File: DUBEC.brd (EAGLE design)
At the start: 40 x 21.4 mm, 72 parts

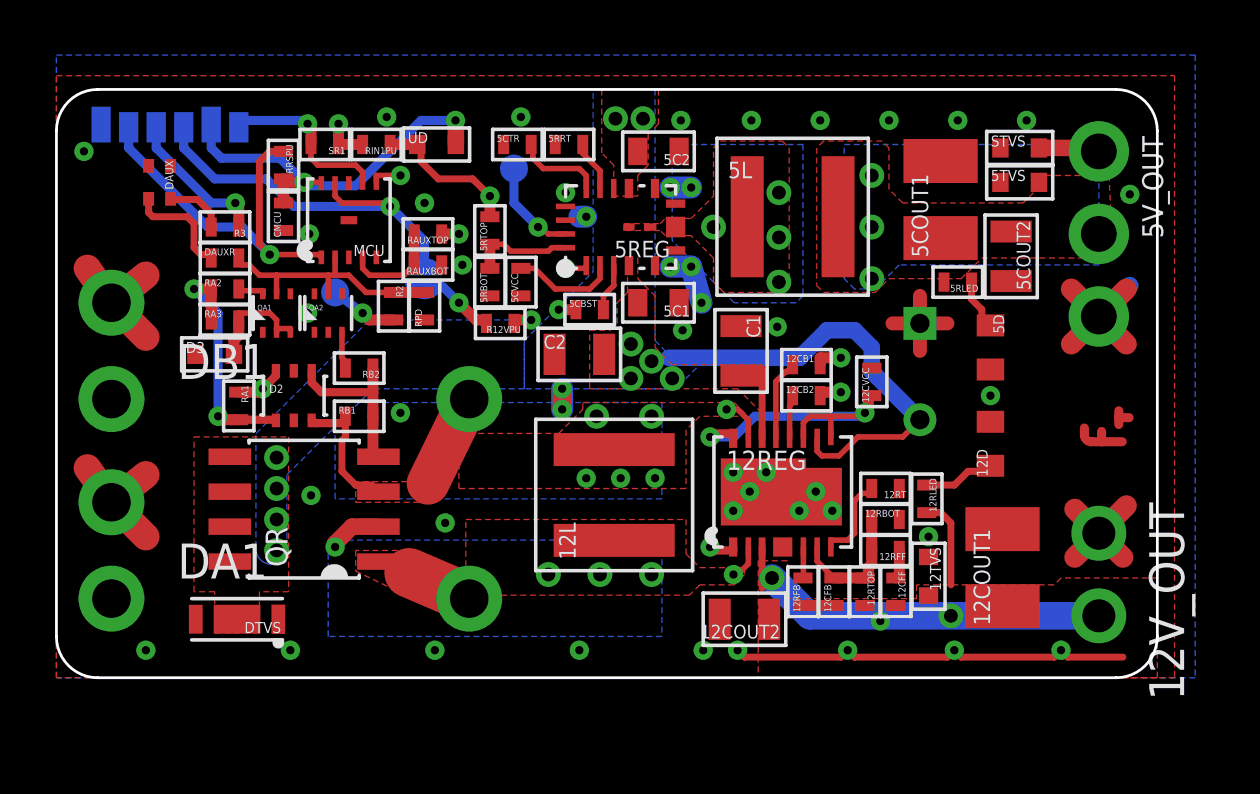
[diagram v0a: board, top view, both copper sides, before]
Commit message: Bored wanking
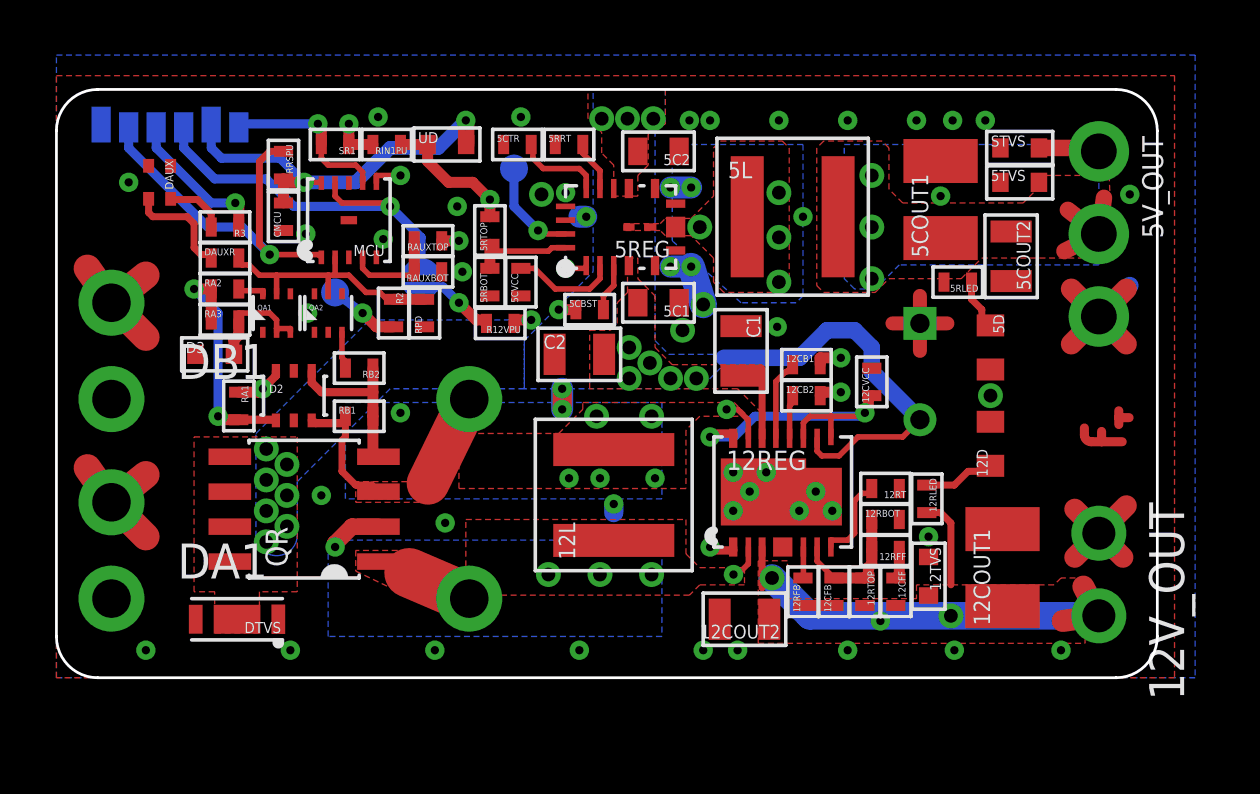
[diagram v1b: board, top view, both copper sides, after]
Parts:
- C1, C2: value 22uF -> (none)
- moved RIN1PU 0.38 mm to (12.0, 19.4)
- moved SR1 0.38 mm to (10.1, 19.4)
- moved UD 0.38 mm to (14.2, 19.4)
- moved R2 0.25 mm to (12.2, 13.2)
- moved RAUXBOT 0.25 mm to (13.5, 14.8)
- moved RAUXTOP 0.25 mm to (13.5, 15.9)
- moved RPD 0.25 mm to (13.4, 13.2)
- moved SJ1 0.12 mm to (13.2, 14.5)
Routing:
- net GND: track 45.5 -> 31.2 mm, vias 46 -> 52
- net 35V: track 38.9 -> 48.2 mm, vias 10 -> 15
- net 5V: track 39.5 -> 43.5 mm
- net 12V: track 30.2 -> 32.7 mm
- net 12V_SW1: track 9.70 -> 8.32 mm

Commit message: Tweaks
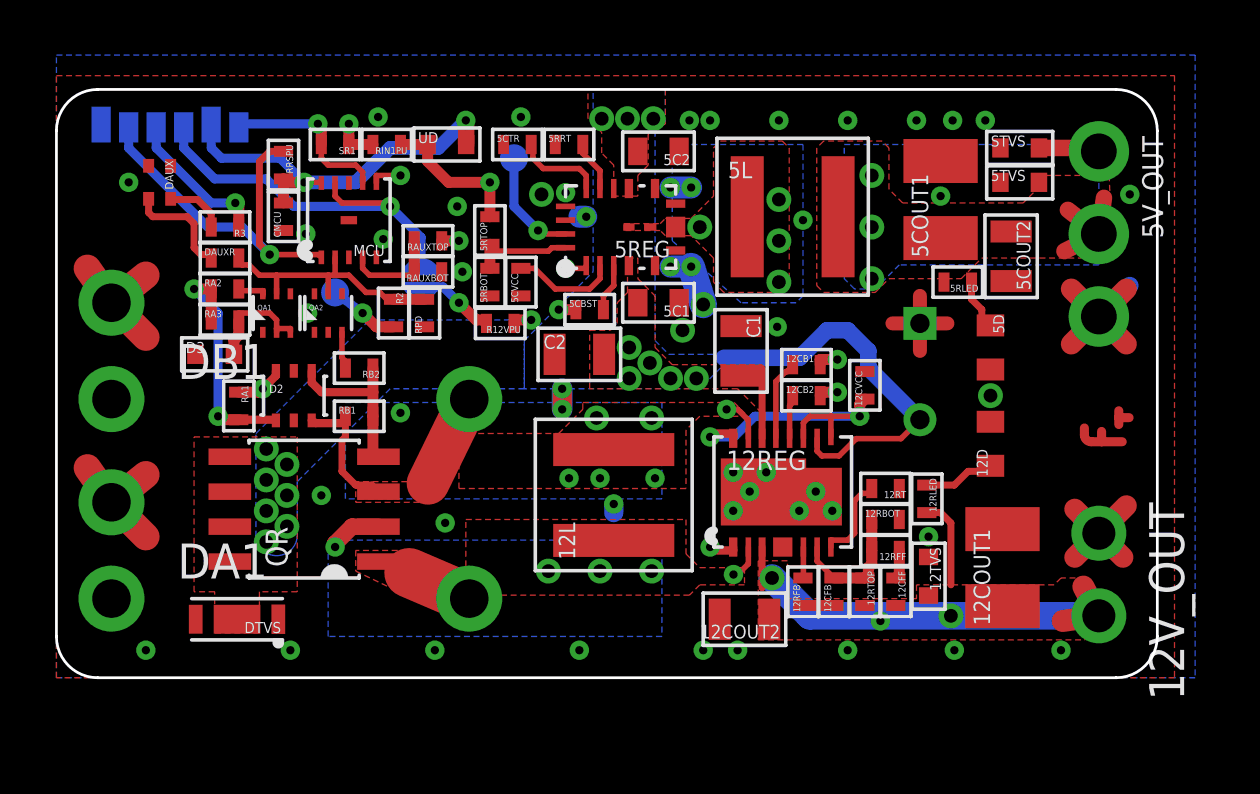
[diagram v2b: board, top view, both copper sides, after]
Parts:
- moved 5V_PG 0.38 mm to (16.6, 18.9)
- moved 12CVCC 0.28 mm to (29.4, 10.6)
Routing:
- net 5V: track 43.5 -> 44.6 mm
- net 12VCC: track 11.5 -> 11.0 mm
